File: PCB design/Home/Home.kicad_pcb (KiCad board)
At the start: 2 copper layers, 119.4 x 127 mm, 17 parts, among them J1 Fan, J2 LCD, J3 EM LOCK, J4 ACS712 Signal, J5 Power In, J7 RFID, J8 RFID, J9 LCD, U1 ACS712, U3 DHT11, U5 PIR, U6 MQ2

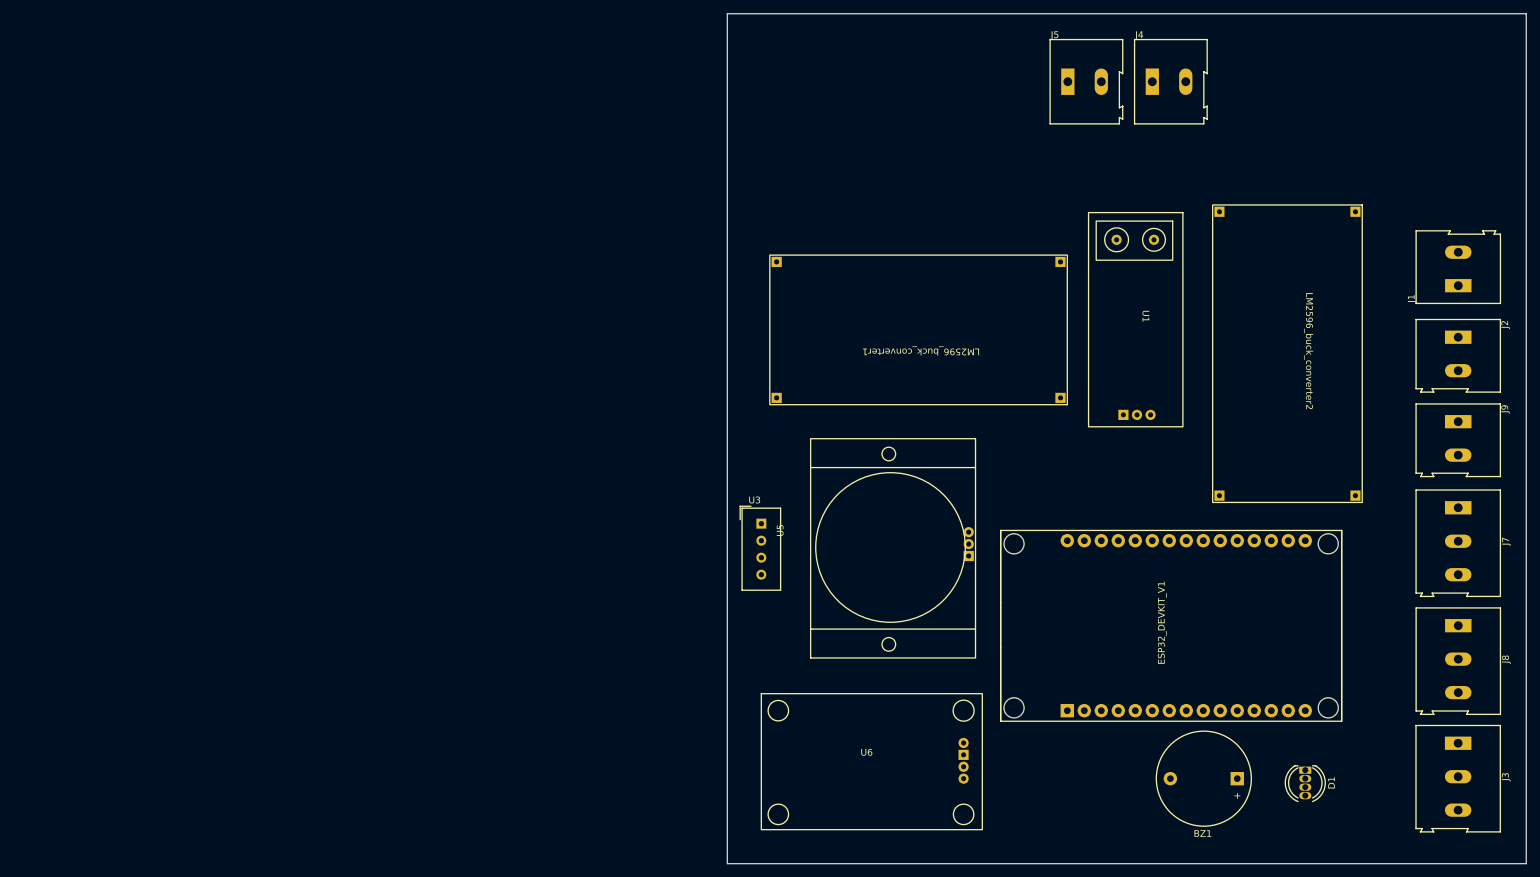
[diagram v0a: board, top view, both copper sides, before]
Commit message: PCB routed
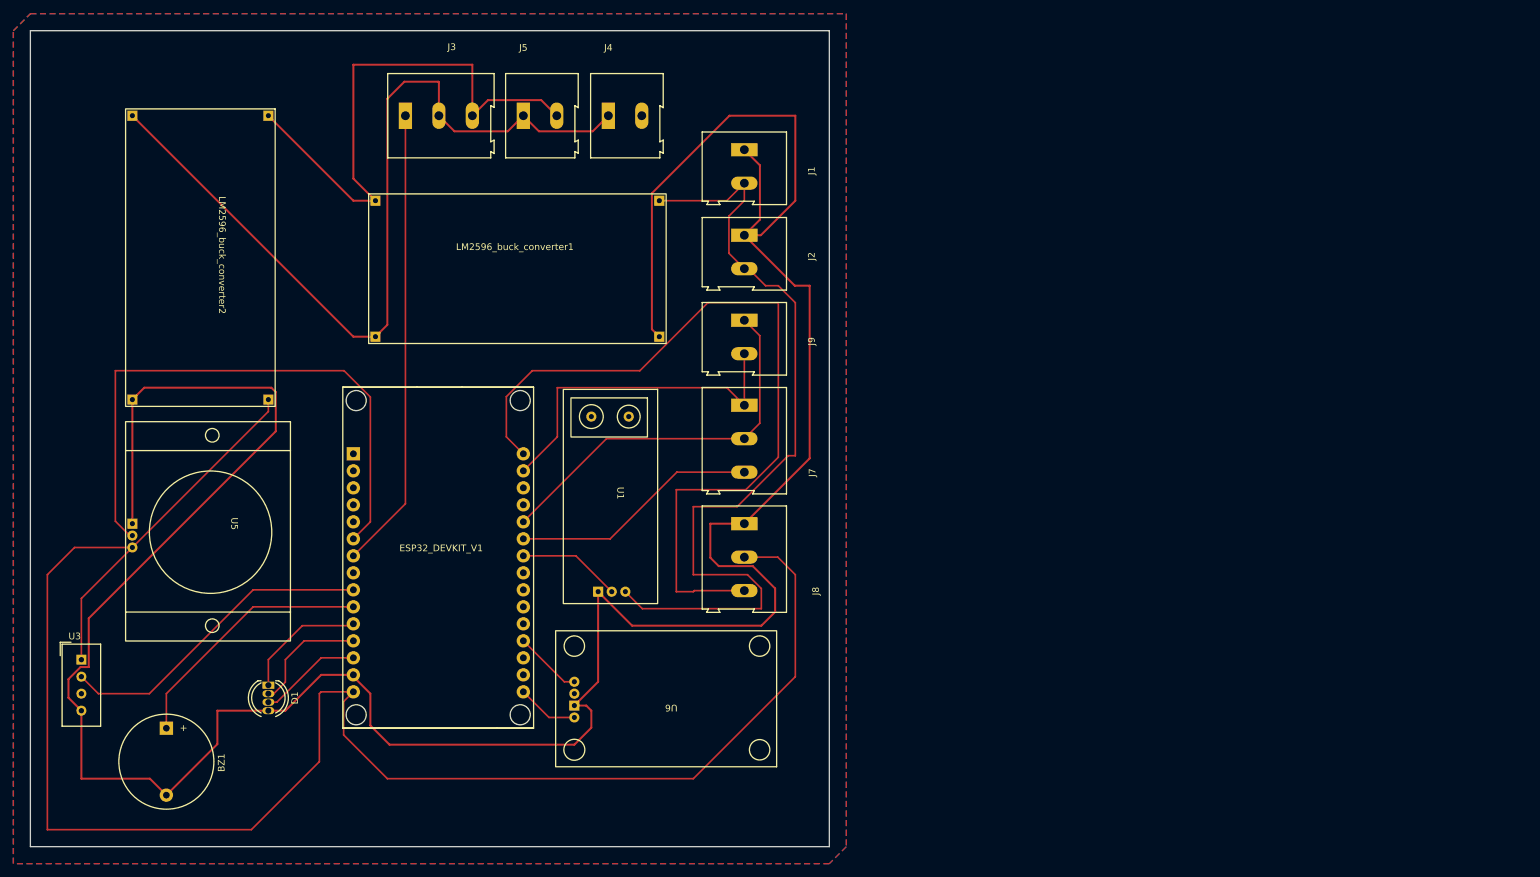
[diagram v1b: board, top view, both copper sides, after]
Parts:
- moved J3 183.1 mm to (111.9, 40.6), turned to 0 degrees
- moved LM2596_buck_converter2 163.1 mm to (92.5, 39.6)
- moved BZ1 160.2 mm to (76.2, 132.2), turned to -90 degrees
- moved D1 155.5 mm to (91.4, 125.7)
- moved ESP32_DEVKIT_V1 110.0 mm to (116.8, 106.7), turned to 0 degrees
- moved LM2596_buck_converter1 109.0 mm to (106.4, 52.3), turned to 0 degrees
- moved J1 108.6 mm to (162.6, 45.7), turned to -90 degrees
- moved J7 107.8 mm to (162.6, 83.9)
- moved J8 107.8 mm to (162.6, 101.6)
- moved J2 107.8 mm to (162.6, 58.5)
- moved J9 107.7 mm to (162.6, 71.2)
- moved U3 103.6 mm to (63.5, 121.9)
- moved U5 88.5 mm to (89.4, 106.4), turned to -90 degrees
- moved U1 82.8 mm to (149.6, 81.5)
- moved J5 81.5 mm to (129.5, 40.6)
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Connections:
- ESP32_DEVKIT_V1 pad 10: unconnected-(ESP32_DEVKIT_V1-GPIO27-Pad10) -> BUZZ
- ESP32_DEVKIT_V1 pad 11: BLUE -> RED
- ESP32_DEVKIT_V1 pad 12: GREEN -> BLUE
- ESP32_DEVKIT_V1 pad 13: RED -> GREEN
- ESP32_DEVKIT_V1 pad 21: DHT -> unconnected-(ESP32_DEVKIT_V1-GPIO16/RXD_2-Pad21)
- ESP32_DEVKIT_V1 pad 24: RELAY -> ACS
- ESP32_DEVKIT_V1 pad 26: unconnected-(ESP32_DEVKIT_V1-GPIO21/SDA-Pad26) -> SDA
- ESP32_DEVKIT_V1 pad 4: ACS -> unconnected-(ESP32_DEVKIT_V1-GPIO34-Pad4)
- ESP32_DEVKIT_V1 pad 7: SDA -> RELAY
- ESP32_DEVKIT_V1 pad 8: BUZZ -> unconnected-(ESP32_DEVKIT_V1-GPIO25-Pad8)
- ESP32_DEVKIT_V1 pad 9: unconnected-(ESP32_DEVKIT_V1-GPIO26-Pad9) -> DHT
- J1 pad 1: 5V -> GND
- J1 pad 2: -5V -> +5V
- J2 pad 1: 5V -> GND
- J2 pad 2: -5V -> +5V
- J3 pad 1: 12V -> RELAY
- J3 pad 2: GND -> -12V
- J3 pad 3: RELAY -> +12V
- J4 pad 1: IP+ -> -12V
- J4 pad 2: -12V -> unconnected-(J4-Pin_2-Pad2)
- J5 pad 1: +12V -> -12V
- J5 pad 2: -12V -> +12V
- J7 pad 1: MISO -> SCK
- J7 pad 2: MOSI -> SDA
- J7 pad 3: SCK -> MISO
- J8 pad 1: SDA -> GND
- J8 pad 2: 3.3V -> +3.3V
- J8 pad 3: GND -> MOSI
- U3 pad 1: 3V3 -> +3.3V
- U5 pad 3: 3V3 -> +3.3V
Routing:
- net GND: track 0.00 -> 425.1 mm
- net +3.3V: track 0.00 -> 270.6 mm
- net -12V: track 0.00 -> 129.3 mm
- net +5V: track 0.00 -> 125.0 mm
- net MOSI: track 0.00 -> 121.9 mm
- net PIR: track 0.00 -> 88.6 mm
- net +12V: track 0.00 -> 82.9 mm
- net RELAY: track 0.00 -> 69.0 mm
- net SDA: track 0.00 -> 57.8 mm
- net SCK: track 0.00 -> 51.3 mm
- net DHT: track 0.00 -> 48.1 mm
- net BUZZ: track 0.00 -> 38.5 mm
- net MISO: track 0.00 -> 37.1 mm
- net RED: track 0.00 -> 18.6 mm
- net BLUE: track 0.00 -> 17.9 mm
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- added copper zone on B.Cu, net GND
- added copper zone on F.Cu, net GND
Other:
- board size 119.4 x 127 mm -> 119.4 x 121.9 mm
